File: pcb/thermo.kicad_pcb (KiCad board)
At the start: 2 copper layers, 29 parts, among them J1 DB15_Female, J2 Barrel_Jack, U1 BME280

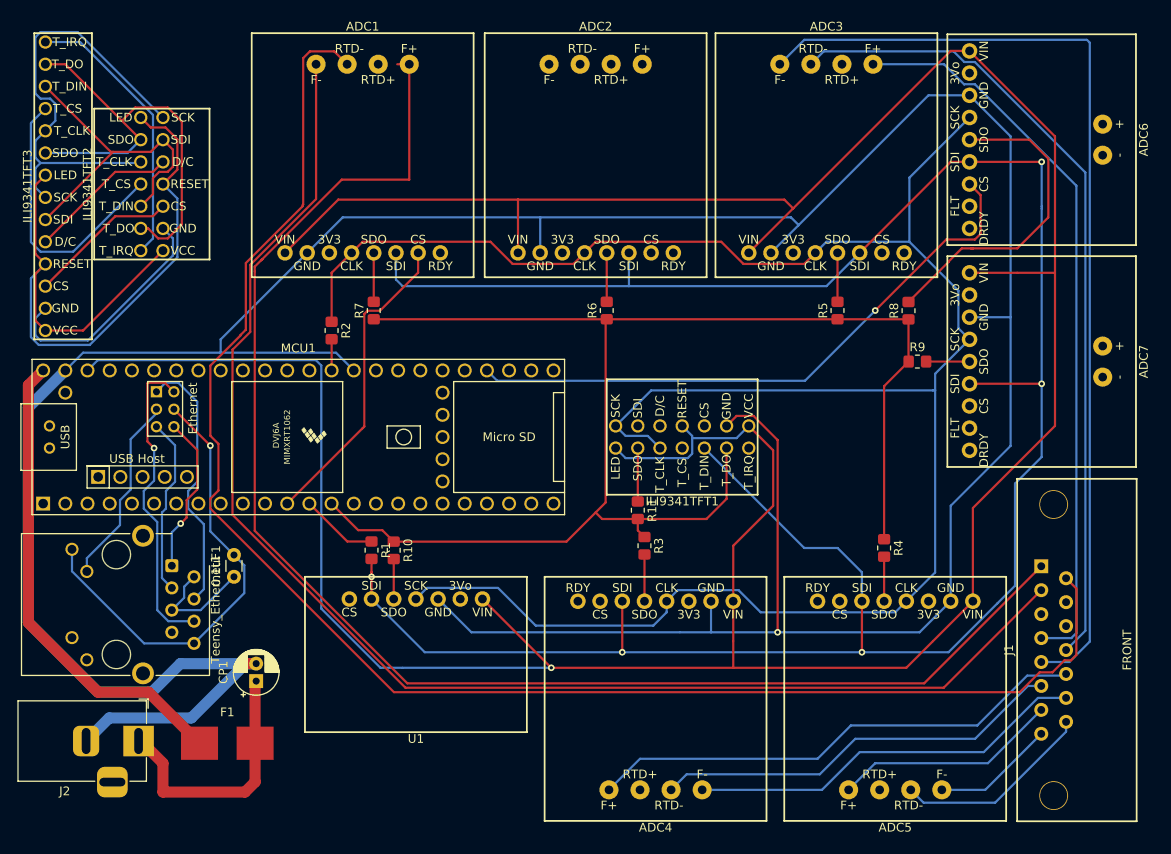
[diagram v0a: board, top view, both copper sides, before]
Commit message: BM routing attempt
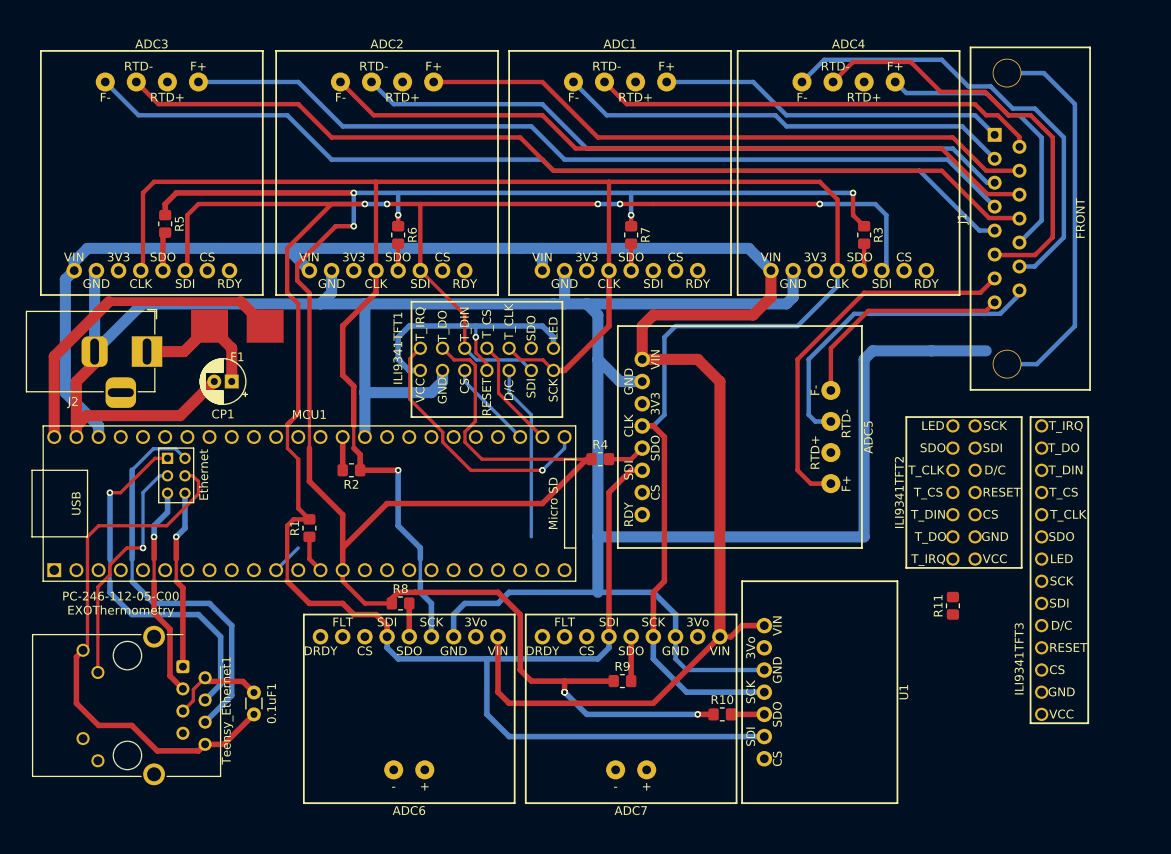
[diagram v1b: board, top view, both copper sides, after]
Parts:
- moved ILI9341TFT3 122.2 mm to (134.6, 123.2)
- moved ILI9341TFT2 99.4 mm to (125.7, 114.3)
- moved ADC6 97.4 mm to (62.2, 139.1), turned to 180 degrees
- moved R5 77.6 mm to (34.3, 83.5), turned to 270 degrees
- moved ADC3 77.2 mm to (32.8, 77.7)
- moved R8 67.1 mm to (61.2, 127.0), turned to 0 degrees
- moved ADC4 64.1 mm to (112.5, 77.7), turned to 0 degrees
- moved ADC7 61.5 mm to (87.6, 139.1), turned to 180 degrees
- moved R9 49.8 mm to (86.6, 135.9)
- moved J1 49.7 mm to (132.1, 83.0)
- moved F1 47.8 mm to (42.6, 95.2), turned to 180 degrees
- moved U1 46.4 mm to (109.2, 137.2), turned to 270 degrees
- moved J2 44.6 mm to (32.2, 98.2)
- moved R3 43.6 mm to (114.3, 84.8)
- moved R10 42.0 mm to (98.1, 139.7), turned to 0 degrees
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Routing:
- net +3V3: track 468.3 -> 244.1 mm
- net Net-(ADC1-Pad10): track 181.6 -> 51.2 mm
- net Net-(ADC1-Pad12): track 169.6 -> 40.1 mm
- net GND: track 417.7 -> 308.3 mm, vias 1 -> 0
- net Net-(ADC1-Pad9): track 160.9 -> 51.9 mm
- net Net-(ADC2-Pad9): track 0.00 -> 83.1 mm
- net Net-(ADC2-Pad10): track 0.00 -> 76.1 mm
- net Net-(ADC2-Pad12): track 0.00 -> 71.3 mm
- net /CS_6: track 70.2 -> 0.00 mm, vias 1 -> 0
- net /SDO: track 220.3 -> 265.0 mm, vias 0 -> 8
- net (no net): track 0.00 -> 44.2 mm
- net /CS_1: track 35.7 -> 0.00 mm
- net Net-(ADC6-Pad5): track 36.9 -> 3.81 mm
- net /CLK: track 300.6 -> 268.6 mm, vias 0 -> 1
- net /SDI: track 306.6 -> 279.4 mm
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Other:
- board text added: "PC-246-112-05-C00 EXOThermometry"
